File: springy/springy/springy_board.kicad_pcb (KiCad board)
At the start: 2 copper layers, 110.5 x 200 mm, 67 parts, among them J5 Synth_power_2x5, U1 TL072, U2 TL074

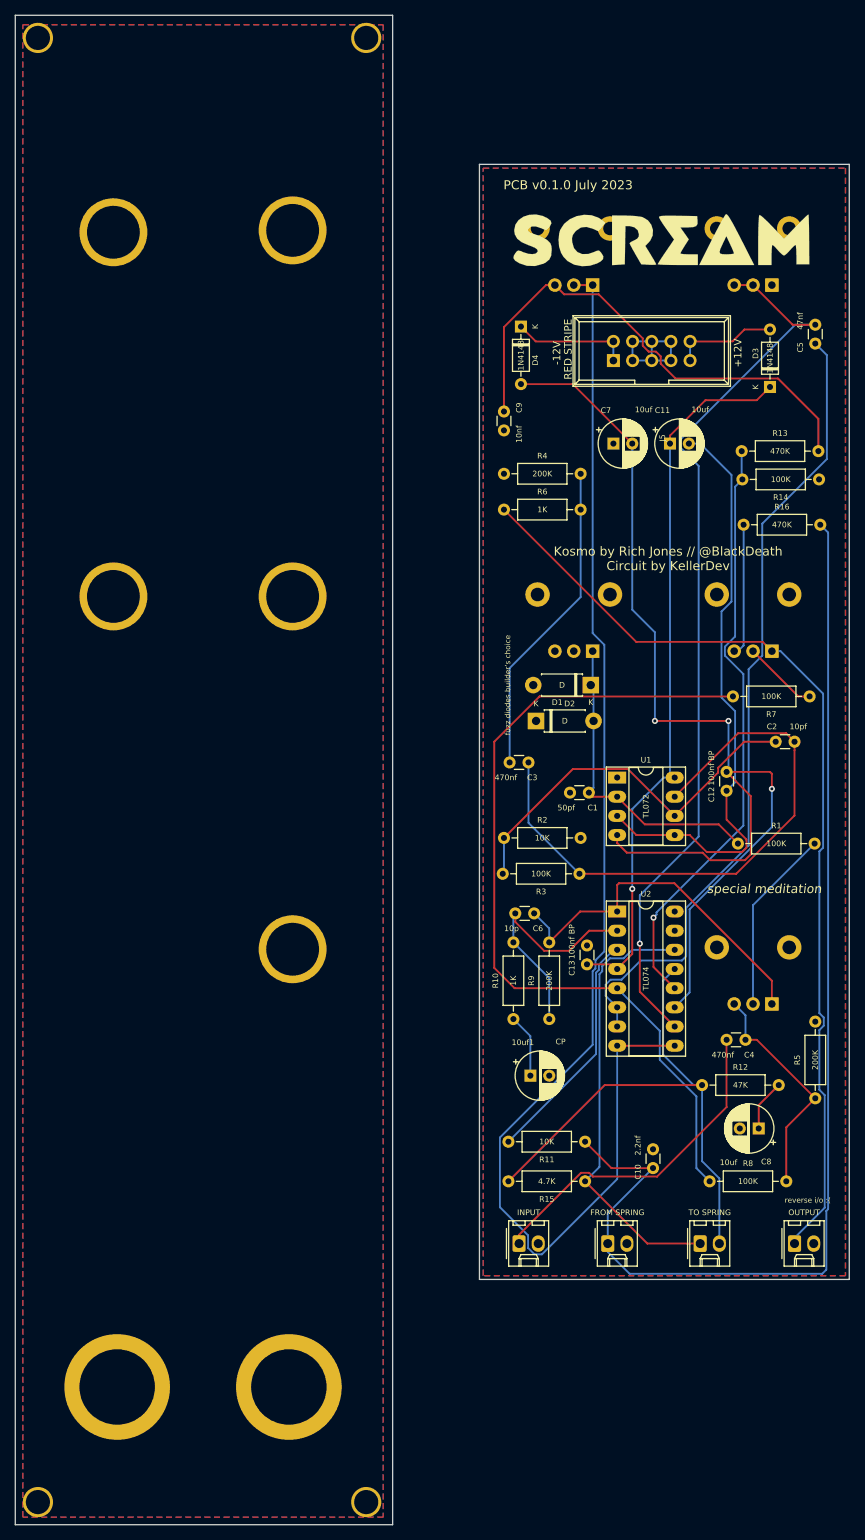
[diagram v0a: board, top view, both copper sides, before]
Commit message: finalize xorcist spring niga
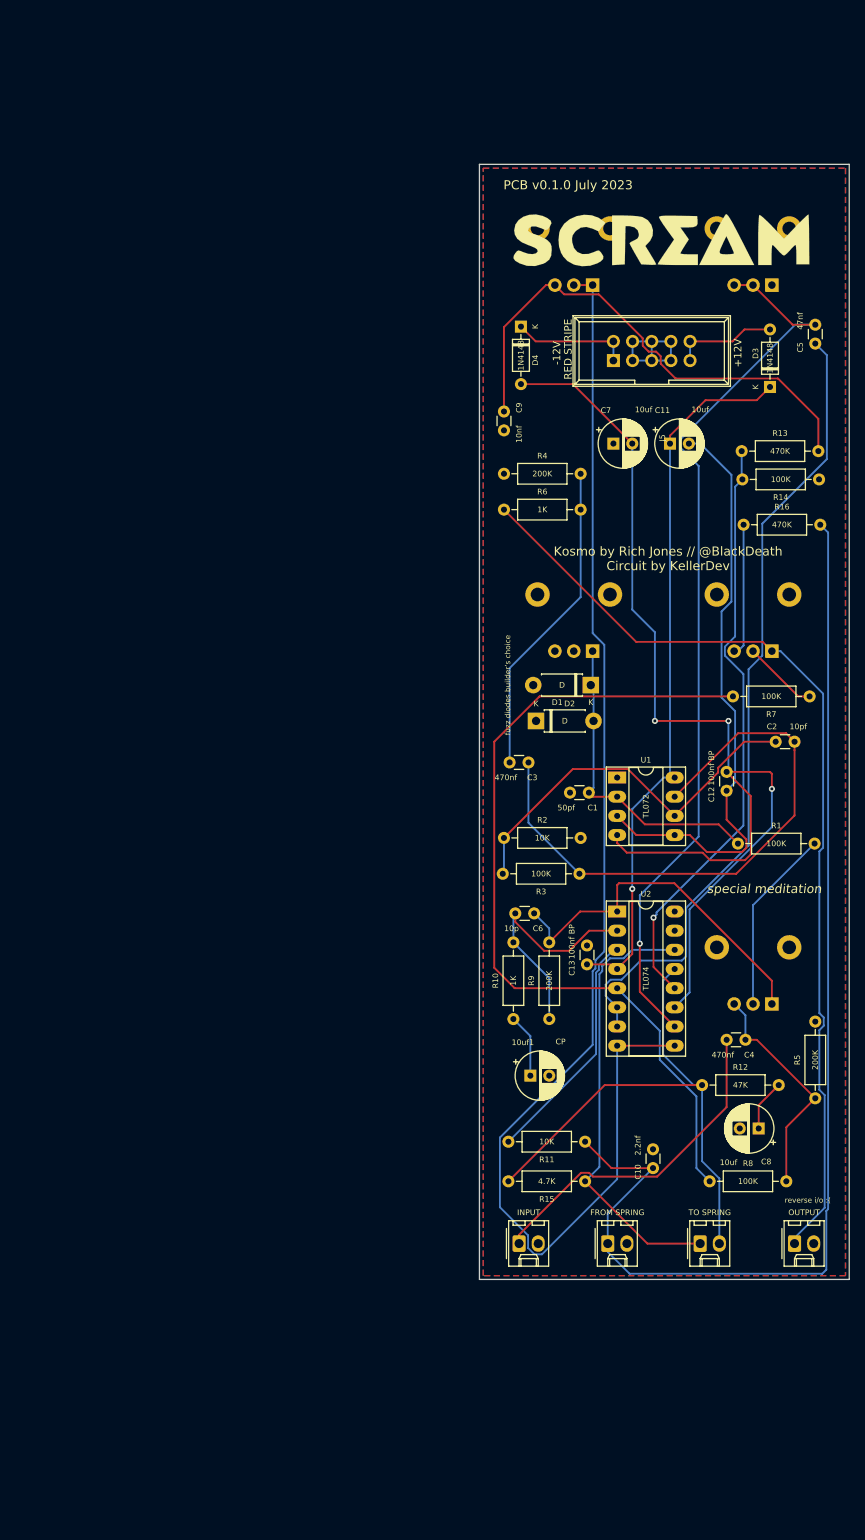
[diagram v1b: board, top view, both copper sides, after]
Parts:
- removed the G*** at (324.0, 102.2)
- removed the G*** at (346.0, 101.5)
- removed the G*** at (343.0, 123.0)
- removed the G*** at (331.0, 66.2)
- removed the G*** at (355.2, 73.0)
- removed the G*** at (331.2, 27.8)
- removed the G*** at (355.0, 27.8)
- removed the G*** at (331.2, -18.5)
- removed the G*** at (355.0, -18.5)
- removed the G*** at (343.0, -59.2)
- removed REF** (x5): Kosmo_Pot_Hole, ao_panel:Kosmo_Pot_Hole
- removed REF** (x2): Kosmo_Jack_Hole, ao_panel:Kosmo_Jack_Hole
- removed REF** (x2): Kosmo_Panel_Dual_Mounting_Holes, ao_panel:Kosmo_Panel_Dual_Mounting_Holes
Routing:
- removed copper zone on B.Cu, net GND
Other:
- board size 110.5 x 200 mm -> 49 x 147.8 mm
